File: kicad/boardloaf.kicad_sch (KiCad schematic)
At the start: 42 parts, among them J1 AudioJack4, J2 AudioJack4, SW1 SW_Push, SW10 SW_Push, SW11 SW_Push, SW12 SW_Push, SW13 SW_Push, SW14 SW_Push, SW15 SW_Push, SW16 SW_Push, SW17 SW_Push, SW18 SW_Push, SW2 SW_Push, SW3 SW_Push, SW4 SW_Push, SW5 SW_Push, SW6 SW_Push, SW7 SW_Push, SW8 SW_Push, SW9 SW_Push, U1 RP2040-Zero

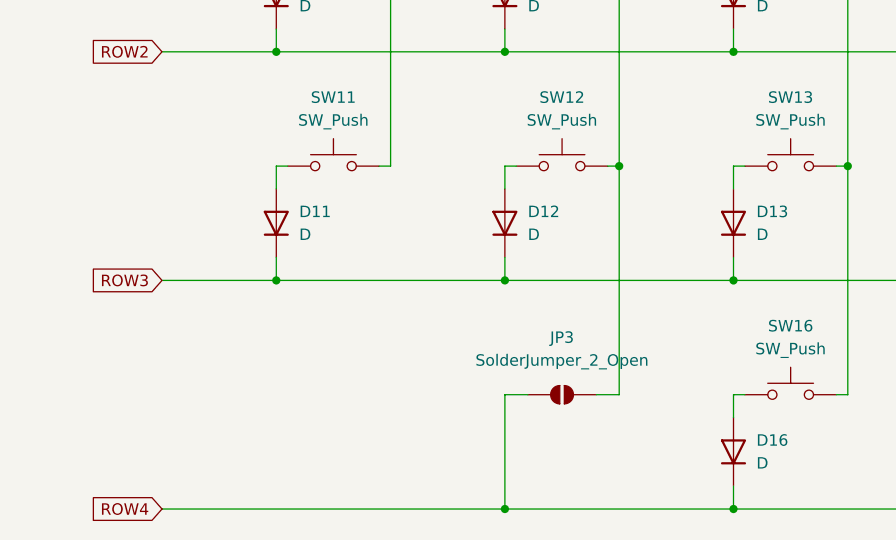
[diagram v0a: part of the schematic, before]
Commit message: get back to once you belong
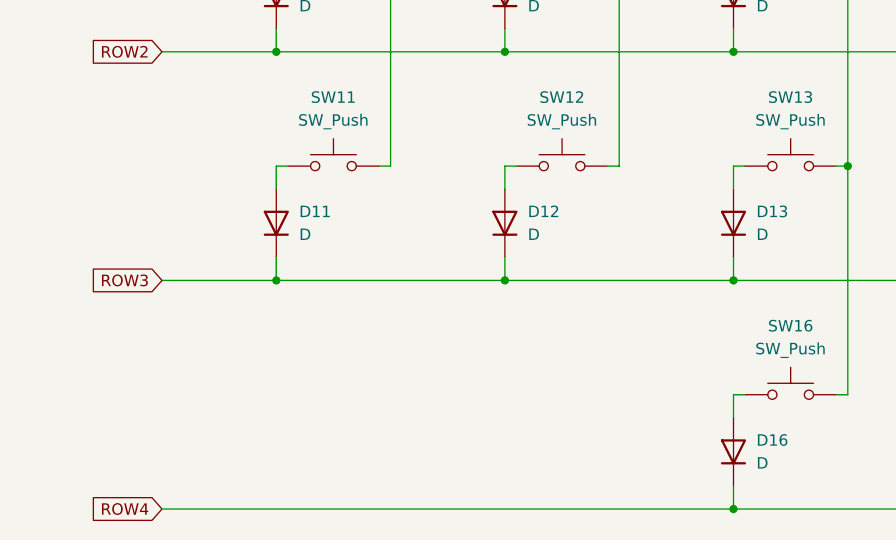
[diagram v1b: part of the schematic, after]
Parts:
- removed JP3: SolderJumper_2_Open, symbol Jumper:SolderJumper_2_Open
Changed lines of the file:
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@@
 	)
 	(junction
-		(at 152.4 88.9)
-		(diameter 0)
-		(color 0 0 0 0)
-	)
-	(junction
 		(at 114.3 101.6)
 		(diameter 0)
@@
 	)
 	(junction
-		(at 139.7 127)
-		(diameter 0)
-		(color 0 0 0 0)
-	)
-	(junction
 		(at 177.8 38.1)
 		(diameter 0)
@@
 	(wire
 		(pts
-			(xy 139.7 114.3) (xy 142.24 114.3)
-		)
-		(stroke
-			(width 0)
-			(type default)
-		)
-	)
-	(wire
-		(pts
 			(xy 139.7 73.66) (xy 139.7 76.2)
 		)
@@
 	(wire
 		(pts
-			(xy 139.7 127) (xy 165.1 127)
-		)
-		(stroke
-			(width 0)
-			(type default)
-		)
-	)
-	(wire
-		(pts
 			(xy 165.1 99.06) (xy 165.1 101.6)
 		)
@@
 	(wire
 		(pts
-			(xy 139.7 114.3) (xy 139.7 127)
-		)
-		(stroke
-			(width 0)
-			(type default)
-		)
-	)
-	(wire
-		(pts
 			(xy 40.64 76.2) (xy 50.8 76.2)
 		)
@@
 	(wire
 		(pts
-			(xy 152.4 114.3) (xy 149.86 114.3)
-		)
-		(stroke
-			(width 0)
-			(type default)
-		)
-	)
-	(wire
-		(pts
 			(xy 60.96 83.82) (xy 59.69 83.82)
 		)
@@
 	(wire
 		(pts
-			(xy 152.4 88.9) (xy 152.4 114.3)
-		)
-		(stroke
-			(width 0)
-			(type default)
-		)
-	)
-	(wire
-		(pts
 			(xy 176.53 114.3) (xy 177.8 114.3)
 		)
@@
 	(wire
 		(pts
-			(xy 101.6 127) (xy 139.7 127)
+			(xy 101.6 127) (xy 165.1 127)
 		)
 		(stroke
@@
 					(unit 1)
 				)
-			)
-		)
-	)
-	(symbol
-		(lib_id "Jumper:SolderJumper_2_Open")
-		(at 146.05 114.3 0)
-		(unit 1)
-		(exclude_from_sim no)
-		(in_bom no)
-		(on_board yes)
-		(dnp no)
-		(fields_autoplaced yes)
-		(property "Reference" "JP3"
-			(at 146.05 107.95 0)
-			(effects
-				(font
-					(size 1.27 1.27)
-				)
-			)
-		)
-		(property "Value" "SolderJumper_2_Open"
-			(at 146.05 110.49 0)
-			(effects
-				(font
-					(size 1.27 1.27)
-				)
-			)
-		)
-		(property "Footprint" ""
-			(at 146.05 114.3 0)
-			(effects
-				(font
-					(size 1.27 1.27)
-				)
-				(hide yes)
-			)
-		)
-		(property "Datasheet" "~"
-			(at 146.05 114.3 0)
-			(effects
-				(font
-					(size 1.27 1.27)
-				)
-				(hide yes)
-			)
-		)
-		(property "Description" "Solder Jumper, 2-pole, open"
-			(at 146.05 114.3 0)
-			(effects
-				(font
-					(size 1.27 1.27)
-				)
-				(hide yes)
-			)
-		)
-		(pin "1"
-		)
-		(pin "2"
-		)
-		(instances
-			(project "boardloaf"
-				(path "/3a093344-253b-4353-a388-64989d9a245c"
-					(reference "JP3")
-					(unit 1)
-				)

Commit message: made jumper for reverse
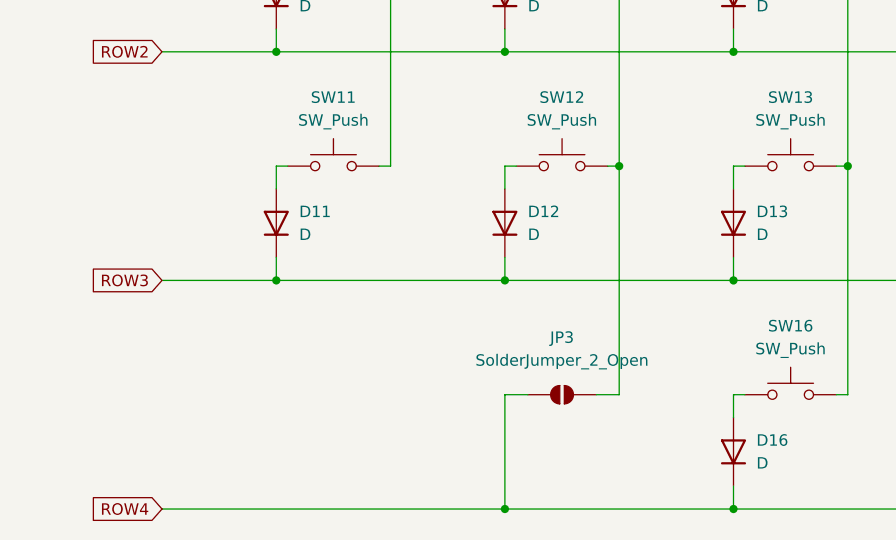
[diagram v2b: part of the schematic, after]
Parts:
- added JP3: SolderJumper_2_Open, symbol Jumper:SolderJumper_2_Open
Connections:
- net COL2: now also JP3.2 (B)
- net ROW4: now also JP3.1 (A)
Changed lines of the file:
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@@
 	)
 	(junction
+		(at 152.4 88.9)
+		(diameter 0)
+		(color 0 0 0 0)
+	)
+	(junction
 		(at 114.3 101.6)
 		(diameter 0)
@@
 	)
 	(junction
+		(at 139.7 127)
+		(diameter 0)
+		(color 0 0 0 0)
+	)
+	(junction
 		(at 177.8 38.1)
 		(diameter 0)
@@
 	(wire
 		(pts
+			(xy 139.7 114.3) (xy 142.24 114.3)
+		)
+		(stroke
+			(width 0)
+			(type default)
+		)
+	)
+	(wire
+		(pts
 			(xy 139.7 73.66) (xy 139.7 76.2)
 		)
@@
 	(wire
 		(pts
+			(xy 139.7 127) (xy 165.1 127)
+		)
+		(stroke
+			(width 0)
+			(type default)
+		)
+	)
+	(wire
+		(pts
 			(xy 165.1 99.06) (xy 165.1 101.6)
 		)
@@
 	(wire
 		(pts
+			(xy 139.7 114.3) (xy 139.7 127)
+		)
+		(stroke
+			(width 0)
+			(type default)
+		)
+	)
+	(wire
+		(pts
 			(xy 40.64 76.2) (xy 50.8 76.2)
 		)
@@
 	(wire
 		(pts
+			(xy 152.4 114.3) (xy 149.86 114.3)
+		)
+		(stroke
+			(width 0)
+			(type default)
+		)
+	)
+	(wire
+		(pts
 			(xy 60.96 83.82) (xy 59.69 83.82)
 		)
@@
 	(wire
 		(pts
+			(xy 152.4 88.9) (xy 152.4 114.3)
+		)
+		(stroke
+			(width 0)
+			(type default)
+		)
+	)
+	(wire
+		(pts
 			(xy 176.53 114.3) (xy 177.8 114.3)
 		)
@@
 	(wire
 		(pts
-			(xy 101.6 127) (xy 165.1 127)
+			(xy 101.6 127) (xy 139.7 127)
 		)
 		(stroke
@@
 					(unit 1)
 				)
+			)
+		)
+	)
+	(symbol
+		(lib_id "Jumper:SolderJumper_2_Open")
+		(at 146.05 114.3 0)
+		(unit 1)
+		(exclude_from_sim no)
+		(in_bom no)
+		(on_board yes)
+		(dnp no)
+		(fields_autoplaced yes)
+		(property "Reference" "JP3"
+			(at 146.05 107.95 0)
+			(effects
+				(font
+					(size 1.27 1.27)
+				)
+			)
+		)
+		(property "Value" "SolderJumper_2_Open"
+			(at 146.05 110.49 0)
+			(effects
+				(font
+					(size 1.27 1.27)
+				)
+			)
+		)
+		(property "Footprint" ""
+			(at 146.05 114.3 0)
+			(effects
+				(font
+					(size 1.27 1.27)
+				)
+				(hide yes)
+			)
+		)
+		(property "Datasheet" "~"
+			(at 146.05 114.3 0)
+			(effects
+				(font
+					(size 1.27 1.27)
+				)
+				(hide yes)
+			)
+		)
+		(property "Description" "Solder Jumper, 2-pole, open"
+			(at 146.05 114.3 0)
+			(effects
+				(font
+					(size 1.27 1.27)
+				)
+				(hide yes)
+			)
+		)
+		(pin "1"
+		)
+		(pin "2"
+		)
+		(instances
+			(project "boardloaf"
+				(path "/3a093344-253b-4353-a388-64989d9a245c"
+					(reference "JP3")
+					(unit 1)
+				)
